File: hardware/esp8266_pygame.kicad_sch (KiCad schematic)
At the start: 27 parts, among them J1 Conn_01x12, J2 Conn_01x12, J3 Conn_01x03, J4 Conn_01x02, J5 Micro_SD_Card, J6 Conn_01x08, Q1 NPN, SW1 SW_Push, SW2 SW_Push, SW3 SW_Push, SW4 SW_Push, SW5 SW_Push, SW6 SW_Push, SW7 SW_Push, SW8 SW_SPST, U1 PCF8574

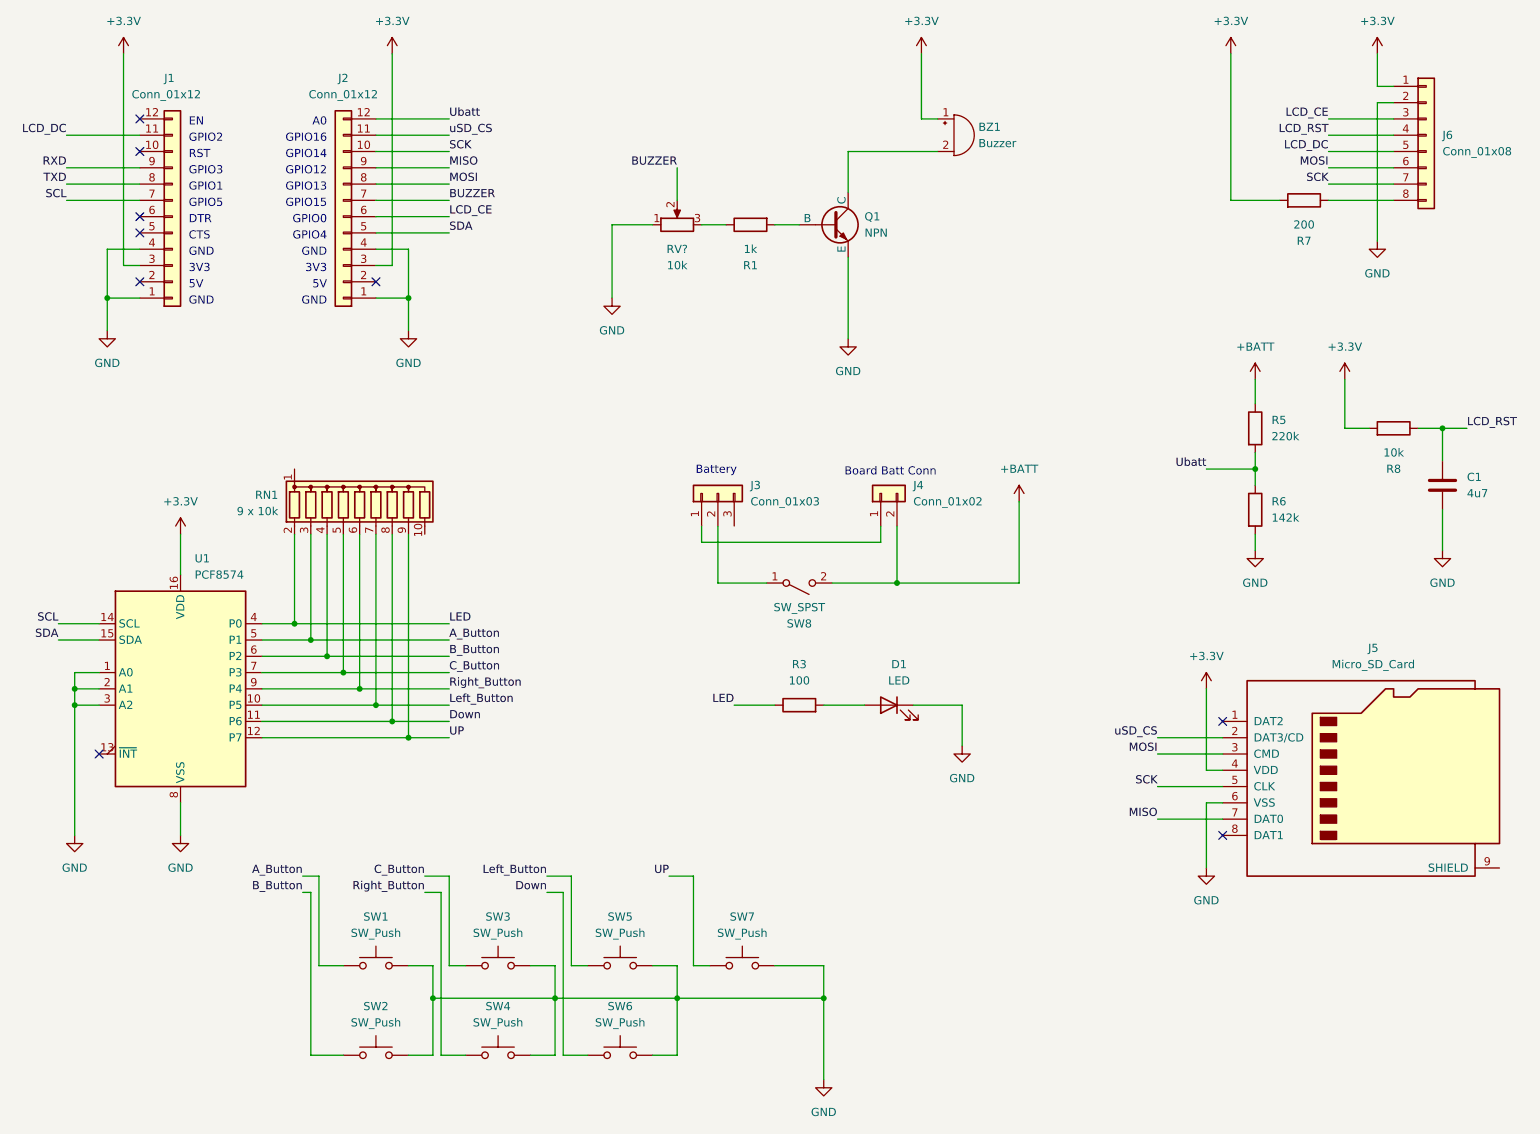
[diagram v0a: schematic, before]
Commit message: New PCB schematic ready
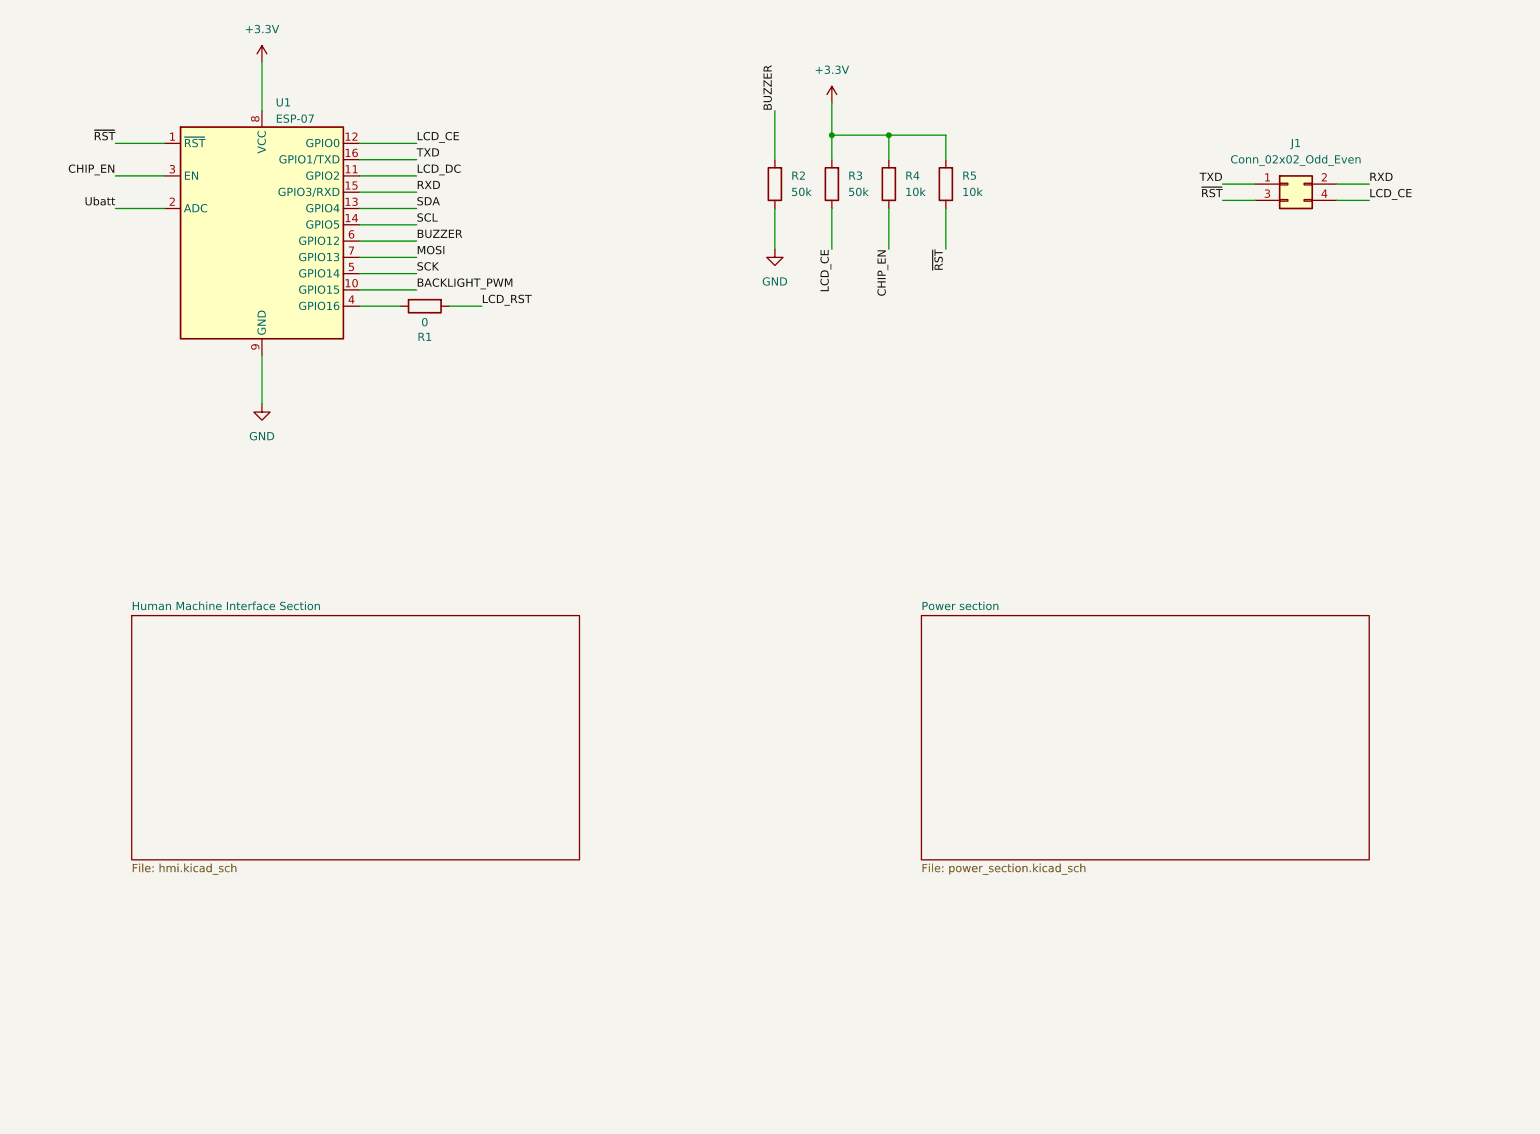
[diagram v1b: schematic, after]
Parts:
- removed BZ1: Buzzer, symbol Device:Buzzer
- removed C1: 4u7, symbol Device:C
- removed D1: LED, symbol Device:LED
- removed J1, J2: Conn_01x12, symbol Connector_Generic:Conn_01x12
- removed J3: Conn_01x03, symbol Connector_Generic:Conn_01x03
- removed J4: Conn_01x02, symbol Connector_Generic:Conn_01x02
- removed J5: Micro_SD_Card, symbol Connector:Micro_SD_Card
- removed J6: Conn_01x08, symbol Connector_Generic:Conn_01x08
- removed Q1: NPN, symbol Simulation_SPICE:NPN
- removed R6: 142k, symbol Device:R
- removed R7: 200, symbol Device:R
- removed R8: 10k, symbol Device:R
- removed RN1: 9 x 10k, Resistor_THT:R_Array_SIP10, symbol Device:R_Network09
- removed RV?: 10k, symbol Device:R_Potentiometer
- removed SW1, SW2, SW3, SW4, SW5, SW6, SW7: SW_Push, symbol Switch:SW_Push
- removed SW8: SW_SPST, symbol Switch:SW_SPST
- removed U1: PCF8574, symbol Interface_Expansion:PCF8574
- added J1: Conn_02x02_Odd_Even, symbol Connector_Generic:Conn_02x02_Odd_Even
- added R2: 50k, symbol Device:R
- added R4: 10k, symbol Device:R
- added U1: ESP-07, RF_Module:ESP-07, symbol RF_Module:ESP-07
- R1: value 1k -> 0
- R3: value 100 -> 50k
- R5: value 220k -> 10k
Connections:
- net LED is gone; now on net LCD_CE: R3.1
- net +3.3V: now also R3.2, R5.2, R4.2, U1.8 (VCC)
- net BUZZER: now also R2.2, U1.6 (GPIO12)
- net GND: now also R2.1, U1.9 (GND)
- net LCD_CE: now also J1.4 (Pin_4), U1.12 (GPIO0)
- net LCD_DC: now also U1.11 (GPIO2)
- net LCD_RST: now also R1.2
- net MOSI: now also U1.7 (GPIO13)
- net RXD: now also J1.2 (Pin_2), U1.15 (GPIO3/RXD)
- net SCK: now also U1.5 (GPIO14)
- net SCL: now also U1.14 (GPIO5)
- net SDA: now also U1.13 (GPIO4)
- net TXD: now also J1.1 (Pin_1), U1.16 (GPIO1/TXD)
- net Ubatt: now also U1.2 (ADC); no longer R5.2
- net at R1.1: now also U1.4 (GPIO16)
- net +BATT renamed ~{RST}
- net ~{RST}: now also J1.3 (Pin_3), U1.1 (~{RST})
- new net BACKLIGHT_PWM: U1.10 (GPIO15)
- new net CHIP_EN: R4.1, U1.3 (EN)
- no-connect marks 9 -> 0
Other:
- added sheet Human Machine Interface Section (hmi.kicad_sch)
- added sheet Power section (power_section.kicad_sch)
- note removed: "3V3"
- note removed: "5V"
- note removed: "A0"
- note removed: "Battery"
- note removed: "Board Batt Conn"
- note removed: "CTS"
- note removed: "DTR"
- note removed: "EN"
- note removed: "GND"
- note removed: "GPIO0"
- note removed: "GPIO1"
- note removed: "GPIO12"
- note removed: "GPIO13"
- note removed: "GPIO14"
- note removed: "GPIO15"
- note removed: "GPIO16"
- note removed: "GPIO2"
- note removed: "GPIO3"
- note removed: "GPIO4"
- note removed: "GPIO5"
- note removed: "RST"
